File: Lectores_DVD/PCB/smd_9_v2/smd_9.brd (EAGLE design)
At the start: 33 x 35.2 mm, 2 parts, among them J1 52793-0970

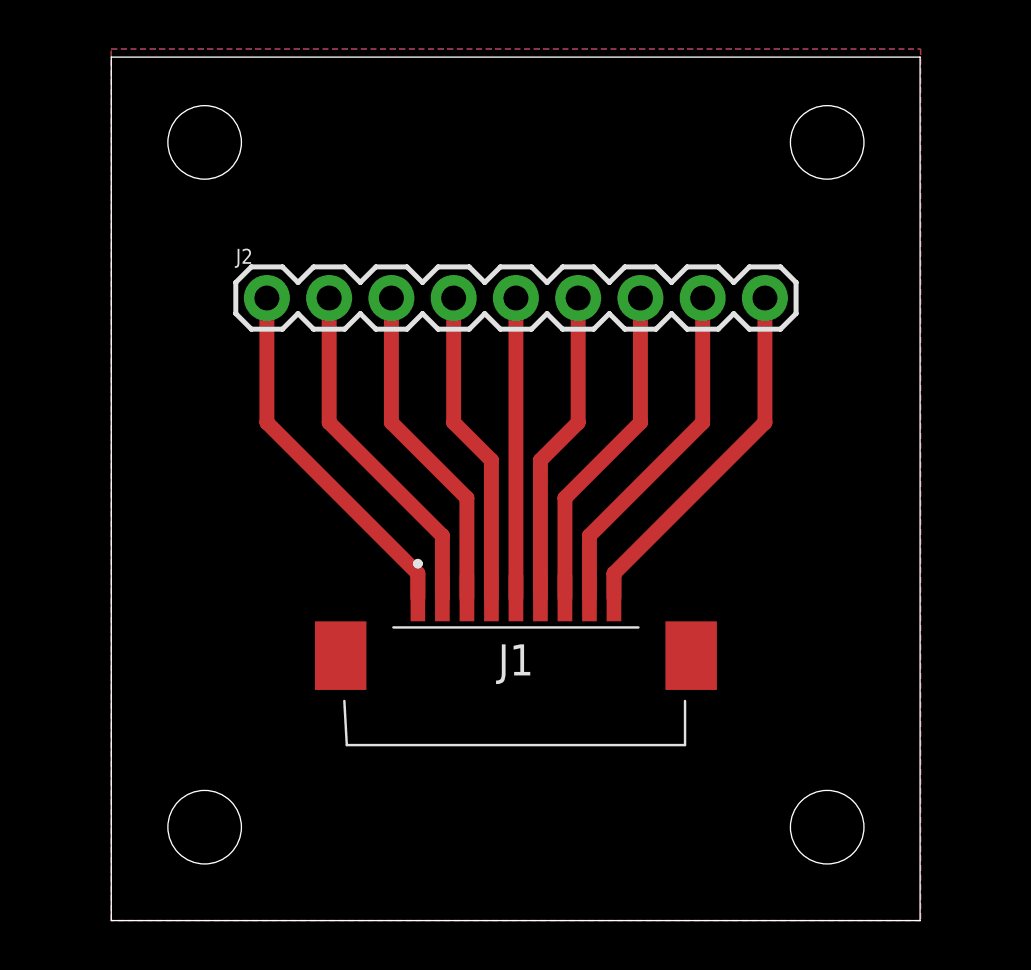
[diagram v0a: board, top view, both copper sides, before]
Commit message: Actualizacion
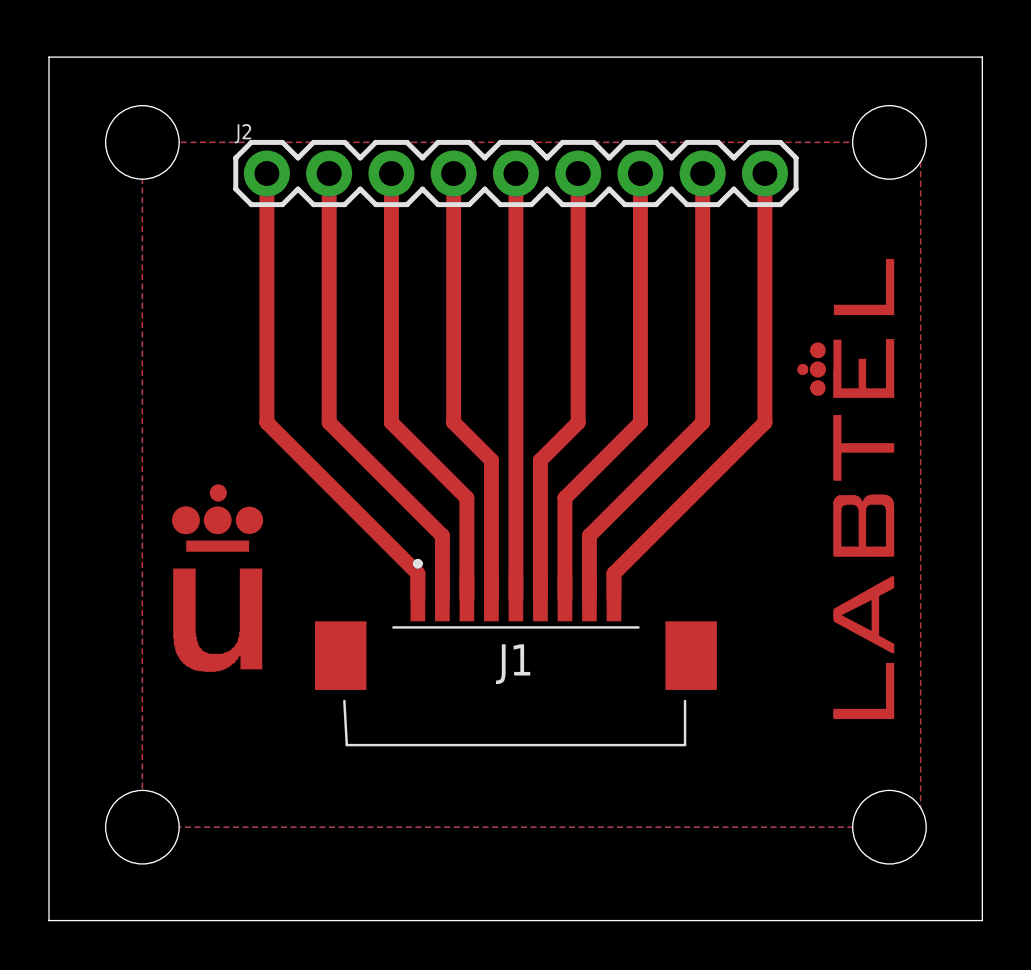
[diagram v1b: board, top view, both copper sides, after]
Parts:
- added U$1: (no value), logos_top:URJC
- added U$2: (no value), logos_top:LABTEL
- moved J2 5.08 mm to (6.35, 30.5)
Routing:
- net N$9: track 14.8 -> 19.9 mm
- net N$8: track 14.2 -> 19.2 mm
- net N$1: track 14.8 -> 19.9 mm
- net N$7: track 13.5 -> 18.6 mm
- net N$6: track 12.9 -> 18.0 mm
- net N$5: track 12.2 -> 17.3 mm
- net N$4: track 12.9 -> 18.0 mm
- net N$3: track 13.5 -> 18.6 mm
- net N$2: track 14.2 -> 19.2 mm
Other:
- board size 33 x 35.2 mm -> 38.1 x 35.2 mm
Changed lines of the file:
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@@
 <board>
 <plain>
-<wire x1="0" y1="0" x2="33" y2="0" width="0" layer="20"/>
-<wire x1="33" y1="0" x2="33" y2="35.23" width="0" layer="20"/>
-<wire x1="33" y1="35.23" x2="0" y2="35.23" width="0" layer="20"/>
-<wire x1="0" y1="35.23" x2="0" y2="0" width="0" layer="20"/>
-<hole x="3.81" y="3.81" drill="3"/>
-<hole x="29.21" y="3.81" drill="3"/>
-<hole x="29.21" y="31.75" drill="3"/>
-<hole x="3.81" y="31.75" drill="3"/>
+<wire x1="-2.54" y1="0" x2="35.54" y2="0" width="0" layer="20"/>
+<wire x1="35.54" y1="0" x2="35.54" y2="35.23" width="0" layer="20"/>
+<wire x1="35.54" y1="35.23" x2="-2.54" y2="35.23" width="0" layer="20"/>
+<wire x1="-2.54" y1="35.23" x2="-2.54" y2="0" width="0" layer="20"/>
+<hole x="1.27" y="3.81" drill="3"/>
+<hole x="31.75" y="3.81" drill="3"/>
+<hole x="31.75" y="31.75" drill="3"/>
+<hole x="1.27" y="31.75" drill="3"/>
 </plain>
 <attributes>
@@
 </class>
 </classes>
-<designrules name="default">
+<designrules name="Fabricacion_interna_microfresadora">
 <description language="de">&lt;b&gt;EAGLE Design Rules&lt;/b&gt;
 &lt;p&gt;
@@
 <param name="mtCopper" value="0.035mm 0.035mm 0.035mm 0.035mm 0.035mm 0.035mm 0.035mm 0.035mm 0.035mm 0.035mm 0.035mm 0.035mm 0.035mm 0.035mm 0.035mm 0.035mm"/>
 <param name="mtIsolate" value="1.5mm 0.15mm 0.2mm 0.15mm 0.2mm 0.15mm 0.2mm 0.15mm 0.2mm 0.15mm 0.2mm 0.15mm 0.2mm 0.15mm 0.2mm"/>
-<param name="mdWireWire" value="6mil"/>
-<param name="mdWirePad" value="6mil"/>
-<param name="mdWireVia" value="6mil"/>
-<param name="mdPadPad" value="6mil"/>
-<param name="mdPadVia" value="6mil"/>
-<param name="mdViaVia" value="6mil"/>
-<param name="mdSmdPad" value="6mil"/>
-<param name="mdSmdVia" value="6mil"/>
-<param name="mdSmdSmd" value="6mil"/>
-<param name="mdViaViaSameLayer" value="6mil"/>
+<param name="mdWireWire" value="12mil"/>
+<param name="mdWirePad" value="12mil"/>
+<param name="mdWireVia" value="12mil"/>
+<param name="mdPadPad" value="12mil"/>
+<param name="mdPadVia" value="12mil"/>
+<param name="mdViaVia" value="12mil"/>
+<param name="mdSmdPad" value="0mil"/>
+<param name="mdSmdVia" value="0mil"/>
+<param name="mdSmdSmd" value="0mil"/>
+<param name="mdViaViaSameLayer" value="8mil"/>
 <param name="mnLayersViaInSmd" value="2"/>
-<param name="mdCopperDimension" value="40mil"/>
-<param name="mdDrill" value="6mil"/>
+<param name="mdCopperDimension" value="12mil"/>
+<param name="mdDrill" value="12mil"/>
 <param name="mdSmdStop" value="0mil"/>
-<param name="msWidth" value="6mil"/>
-<param name="msDrill" value="0.35mm"/>
-<param name="msMicroVia" value="9.99mm"/>
+<param name="msWidth" value="12mil"/>
+<param name="msDrill" value="28mil"/>
+<param name="msMicroVia" value="12mil"/>
 <param name="msBlindViaRatio" value="0.5"/>
 <param name="rvPadTop" value="0.25"/>
@@
 <param name="rvMicroViaOuter" value="0.25"/>
 <param name="rvMicroViaInner" value="0.25"/>
-<param name="rlMinPadTop" value="10mil"/>
+<param name="rlMinPadTop" value="6mil"/>
 <param name="rlMaxPadTop" value="20mil"/>
-<param name="rlMinPadInner" value="10mil"/>
+<param name="rlMinPadInner" value="6mil"/>
 <param name="rlMaxPadInner" value="20mil"/>
-<param name="rlMinPadBottom" value="10mil"/>
+<param name="rlMinPadBottom" value="6mil"/>
 <param name="rlMaxPadBottom" value="20mil"/>
-<param name="rlMinViaOuter" value="8mil"/>
+<param name="rlMinViaOuter" value="6mil"/>
 <param name="rlMaxViaOuter" value="20mil"/>
-<param name="rlMinViaInner" value="8mil"/>
+<param name="rlMinViaInner" value="6mil"/>
 <param name="rlMaxViaInner" value="20mil"/>
 <param name="rlMinMicroViaOuter" value="4mil"/>
@@
 <param name="psTop" value="-1"/>
 <param name="psBottom" value="-1"/>
-<param name="psFirst" value="-1"/>
+<param name="psFirst" value="0"/>
 <param name="psElongationLong" value="100"/>
 <param name="psElongationOffset" value="100"/>
@@
 <param name="srMinRoundness" value="0mil"/>
 <param name="srMaxRoundness" value="0mil"/>
-<param name="slThermalIsolate" value="10mil"/>
+<param name="slThermalIsolate" value="12mil"/>
 <param name="slThermalsForVias" value="0"/>
 <param name="dpMaxLengthDifference" value="10mm"/>
@@
 <attribute name="VALUE" x="16.51" y="10.635" size="1.27" layer="27" align="center"/>
 </element>
-<element name="J2" library="SparkFun-Connectors" package="1X09" value="" x="6.35" y="25.4" smashed="yes">
-<attribute name="NAME" x="5.08" y="26.797" size="0.6096" layer="25" font="vector" ratio="20"/>
-<attribute name="VALUE" x="5.08" y="23.368" size="0.6096" layer="27" font="vector" ratio="20"/>
+<element name="J2" library="SparkFun-Connectors" package="1X09" value="" x="6.35" y="30.48" smashed="yes">
+<attribute name="NAME" x="5.08" y="31.877" size="0.6096" layer="25" font="vector" ratio="20"/>
+<attribute name="VALUE" x="5.08" y="28.448" size="0.6096" layer="27" font="vector" ratio="20"/>
 </element>
+<element name="U$1" library="logos_top" package="URJC" value="" x="2.54" y="10.16" smashed="yes"/>
+<element name="U$2" library="logos_top" package="LABTEL" value="" x="33.02" y="7.62" smashed="yes" rot="R90"/>
 </elements>
 <signals>
@@
 <wire x1="12.51" y1="13.16" x2="12.51" y2="14.16" width="0.6096" layer="1"/>
 <wire x1="12.51" y1="14.16" x2="6.35" y2="20.32" width="0.6096" layer="1"/>
-<wire x1="6.35" y1="20.32" x2="6.35" y2="25.4" width="0.6096" layer="1"/>
+<wire x1="6.35" y1="20.32" x2="6.35" y2="30.48" width="0.6096" layer="1"/>
 </signal>
 <signal name="N$2">
@@
 <wire x1="13.51" y1="13.16" x2="13.51" y2="15.7" width="0.6096" layer="1"/>
 <wire x1="13.51" y1="15.7" x2="8.89" y2="20.32" width="0.6096" layer="1"/>
-<wire x1="8.89" y1="20.32" x2="8.89" y2="25.4" width="0.6096" layer="1"/>
+<wire x1="8.89" y1="20.32" x2="8.89" y2="30.48" width="0.6096" layer="1"/>
 </signal>
 <signal name="N$3">
@@
 <wire x1="14.51" y1="13.16" x2="14.51" y2="17.24" width="0.6096" layer="1"/>
 <wire x1="14.51" y1="17.24" x2="11.43" y2="20.32" width="0.6096" layer="1"/>
-<wire x1="11.43" y1="20.32" x2="11.43" y2="25.4" width="0.6096" layer="1"/>
+<wire x1="11.43" y1="20.32" x2="11.43" y2="30.48" width="0.6096" layer="1"/>
 </signal>
 <signal name="N$4">
@@
 <wire x1="15.51" y1="13.16" x2="15.51" y2="18.78" width="0.6096" layer="1"/>
 <wire x1="15.51" y1="18.78" x2="13.97" y2="20.32" width="0.6096" layer="1"/>
-<wire x1="13.97" y1="20.32" x2="13.97" y2="25.4" width="0.6096" layer="1"/>
+<wire x1="13.97" y1="20.32" x2="13.97" y2="30.48" width="0.6096" layer="1"/>
 </signal>
 <signal name="N$5">
 <contactref element="J1" pad="5"/>
 <contactref element="J2" pad="5"/>
-<wire x1="16.51" y1="13.16" x2="16.51" y2="25.4" width="0.6096" layer="1"/>
+<wire x1="16.51" y1="13.16" x2="16.51" y2="30.48" width="0.6096" layer="1"/>
 </signal>
 <signal name="N$6">
@@
 <wire x1="17.51" y1="13.16" x2="17.51" y2="18.78" width="0.6096" layer="1"/>
 <wire x1="17.51" y1="18.78" x2="19.05" y2="20.32" width="0.6096" layer="1"/>
-<wire x1="19.05" y1="20.32" x2="19.05" y2="25.4" width="0.6096" layer="1"/>
+<wire x1="19.05" y1="20.32" x2="19.05" y2="30.48" width="0.6096" layer="1"/>
 </signal>
 <signal name="N$7">
@@
 <wire x1="18.51" y1="13.16" x2="18.51" y2="17.24" width="0.6096" layer="1"/>
 <wire x1="18.51" y1="17.24" x2="21.59" y2="20.32" width="0.6096" layer="1"/>
-<wire x1="21.59" y1="20.32" x2="21.59" y2="25.4" width="0.6096" layer="1"/>
+<wire x1="21.59" y1="20.32" x2="21.59" y2="30.48" width="0.6096" layer="1"/>
 </signal>
 <signal name="N$8">
@@
 <wire x1="19.51" y1="13.16" x2="19.51" y2="15.7" width="0.6096" layer="1"/>
 <wire x1="19.51" y1="15.7" x2="24.13" y2="20.32" width="0.6096" layer="1"/>
-<wire x1="24.13" y1="20.32" x2="24.13" y2="25.4" width="0.6096" layer="1"/>
+<wire x1="24.13" y1="20.32" x2="24.13" y2="30.48" width="0.6096" layer="1"/>
 </signal>
 <signal name="N$9">
@@
 <wire x1="20.51" y1="13.16" x2="20.51" y2="14.16" width="0.6096" layer="1"/>
 <wire x1="20.51" y1="14.16" x2="26.67" y2="20.32" width="0.6096" layer="1"/>
-<wire x1="26.67" y1="20.32" x2="26.67" y2="25.4" width="0.6096" layer="1"/>
+<wire x1="26.67" y1="20.32" x2="26.67" y2="30.48" width="0.6096" layer="1"/>
 </signal>
 <signal name="GND">
 <polygon width="0.6096" layer="16">
-<vertex x="0" y="35.56"/>
-<vertex x="33.02" y="35.56"/>
-<vertex x="33.02" y="0"/>
-<vertex x="0" y="0"/>
+<vertex x="1.27" y="31.75"/>
+<vertex x="33.02" y="31.75"/>
+<vertex x="33.02" y="3.81"/>
+<vertex x="1.27" y="3.81"/>
 </polygon>
 <polygon width="0.6096" layer="1">
-<vertex x="0" y="35.56"/>
-<vertex x="33.02" y="35.56"/>
-<vertex x="33.02" y="0"/>
-<vertex x="0" y="0"/>
+<vertex x="1.27" y="31.75"/>
+<vertex x="33.02" y="31.75"/>
+<vertex x="33.02" y="3.81"/>
+<vertex x="1.27" y="3.81"/>
 </polygon>
 </signal>
@@
 <mfgpreviewcolor name="substratecolor" color="0xFF786E46"/>
 </mfgpreviewcolors>
+<errors>
+</errors>
 </board>
 </drawing>
